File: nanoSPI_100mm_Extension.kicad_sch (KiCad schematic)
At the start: 2 parts, among them J1 FPC contacts 0.3mm

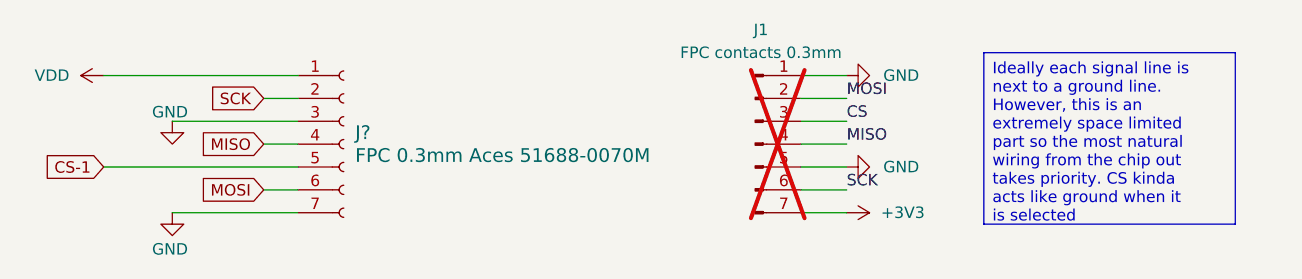
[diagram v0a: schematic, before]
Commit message: Finished Schematic
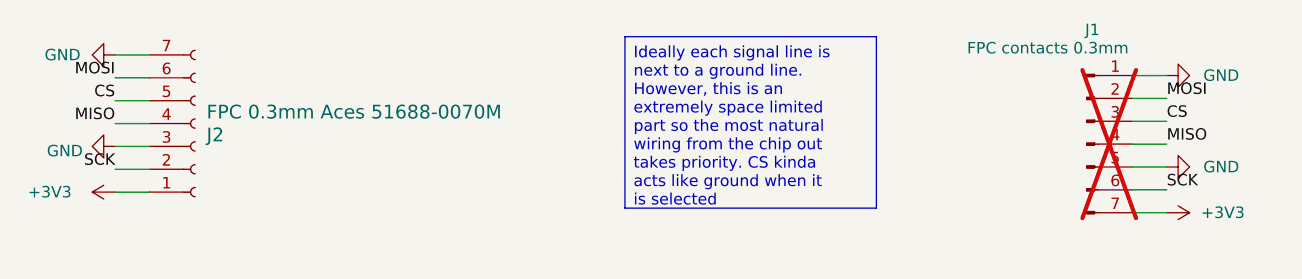
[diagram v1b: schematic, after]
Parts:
- gave numbers to parts that had none: 1
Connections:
- net CS-1 is gone; now on net CS: J2.5 (Pin_5)
- net VDD is gone; now on net +3V3: J2.1 (Pin_1)
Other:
- moved on the sheet: J1, J2
